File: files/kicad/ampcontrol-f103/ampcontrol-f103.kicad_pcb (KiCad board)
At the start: 2 copper layers, 77.2 x 42.7 mm, 63 parts, among them J1 SP, J10 Buttons, J11 Encoder, J12 LCD_CTRL, J13 SPI, J14 I2C, J15 I2C, J16 I2C, J2 MUTE_STBY, J3 UART1, J4 USB, J5 UART2, J6 UART3, J7 RC, J8 LCD_DATA, J9 5V, Q1 BSS138, SW1 Reset, U1 MCP602, U2 STM32F103CBTx, U3 AMS1117-3.3, Y1 8MHz, Y2 32768

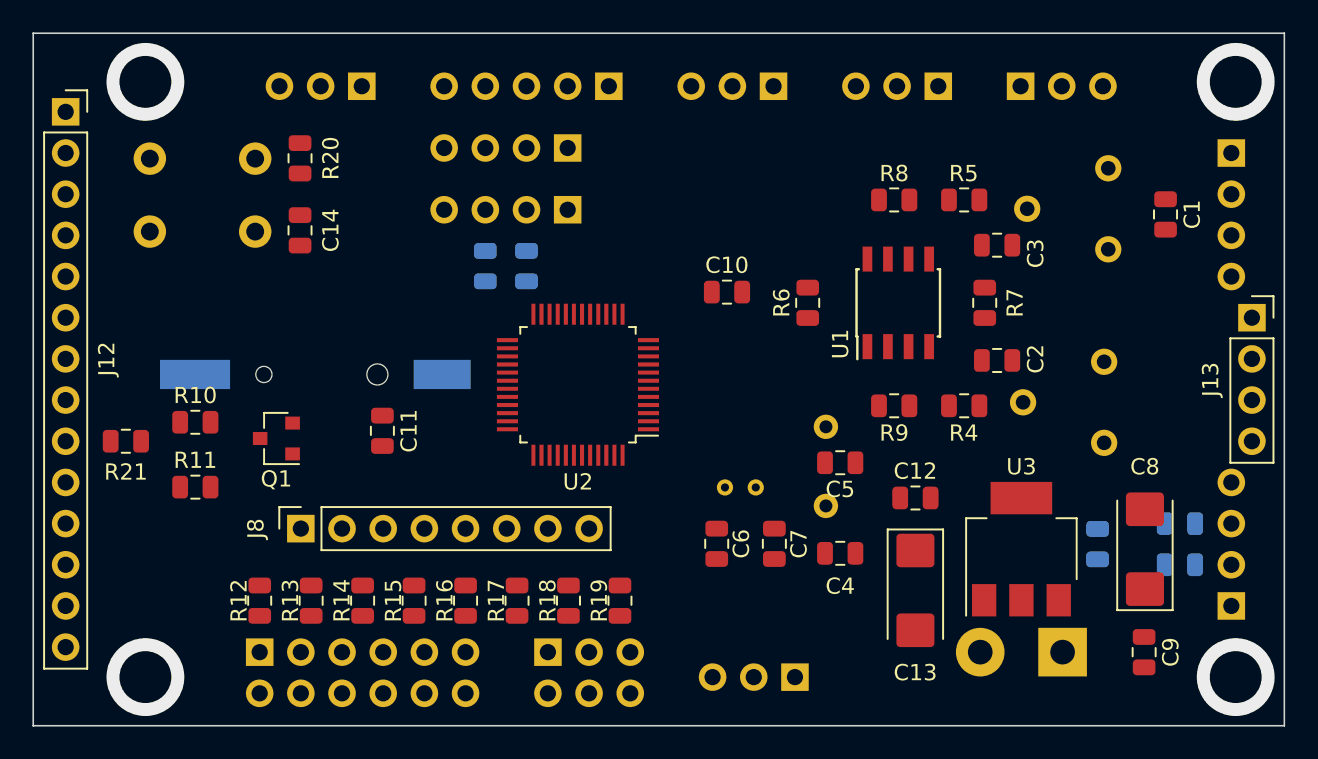
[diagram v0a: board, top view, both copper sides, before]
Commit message: Test PCB layout
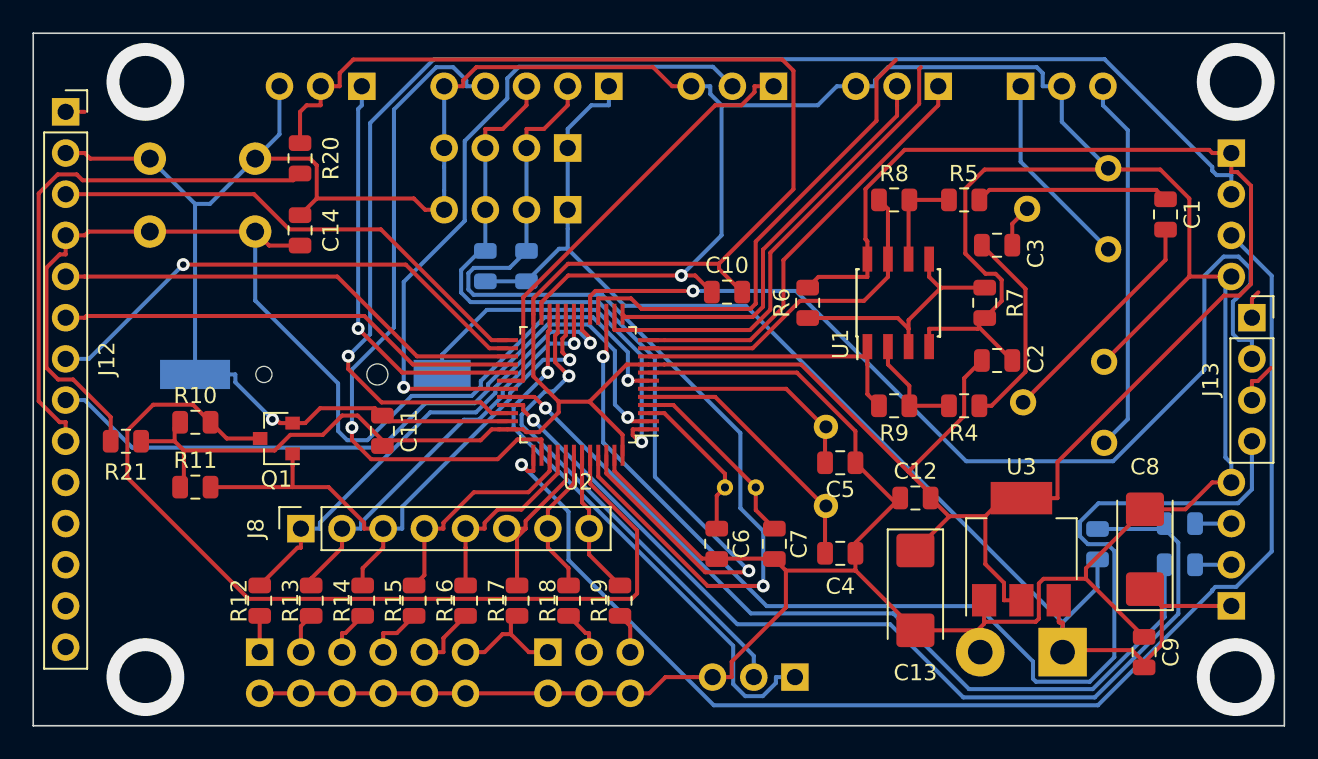
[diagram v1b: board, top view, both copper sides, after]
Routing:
- net GNDD: track 0.00 -> 326.6 mm, vias 0 -> 2
- net +3V3: track 0.00 -> 224.3 mm
- net /MUTE: track 0.00 -> 85.7 mm, vias 0 -> 1
- net +5V: track 0.00 -> 83.1 mm
- net /STBY: track 0.00 -> 80.5 mm, vias 0 -> 1
- net /SD_SCK: track 0.00 -> 71.2 mm, vias 0 -> 1
- net /NRST: track 0.00 -> 70.3 mm, vias 0 -> 1
- net /SD_MOSI: track 0.00 -> 62.3 mm, vias 0 -> 1
- net /SCL: track 0.00 -> 61.8 mm, vias 0 -> 1
- net /USB_DP: track 0.00 -> 61.2 mm, vias 0 -> 1
- net /BOOT0: track 0.00 -> 57.0 mm
- net /SDA: track 0.00 -> 56.8 mm, vias 0 -> 1
- net /USB_DM: track 0.00 -> 53.1 mm, vias 0 -> 1
- net /BCKL: track 0.00 -> 44.9 mm, vias 0 -> 1
- net /RX1: track 0.00 -> 42.8 mm, vias 0 -> 1
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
